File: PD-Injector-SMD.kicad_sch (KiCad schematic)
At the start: 10 parts

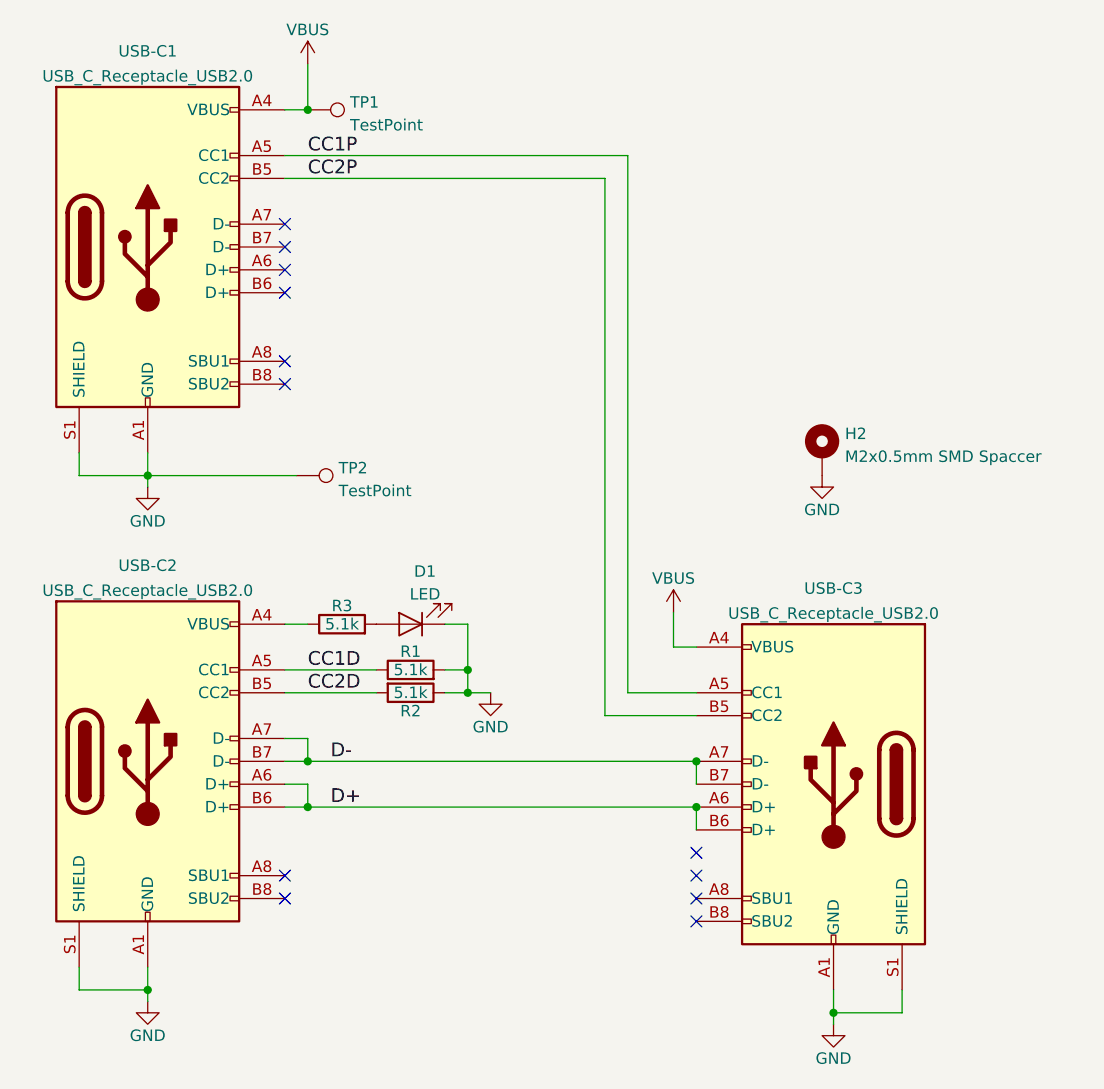
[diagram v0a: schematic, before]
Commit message: Update readme, minor mucking about
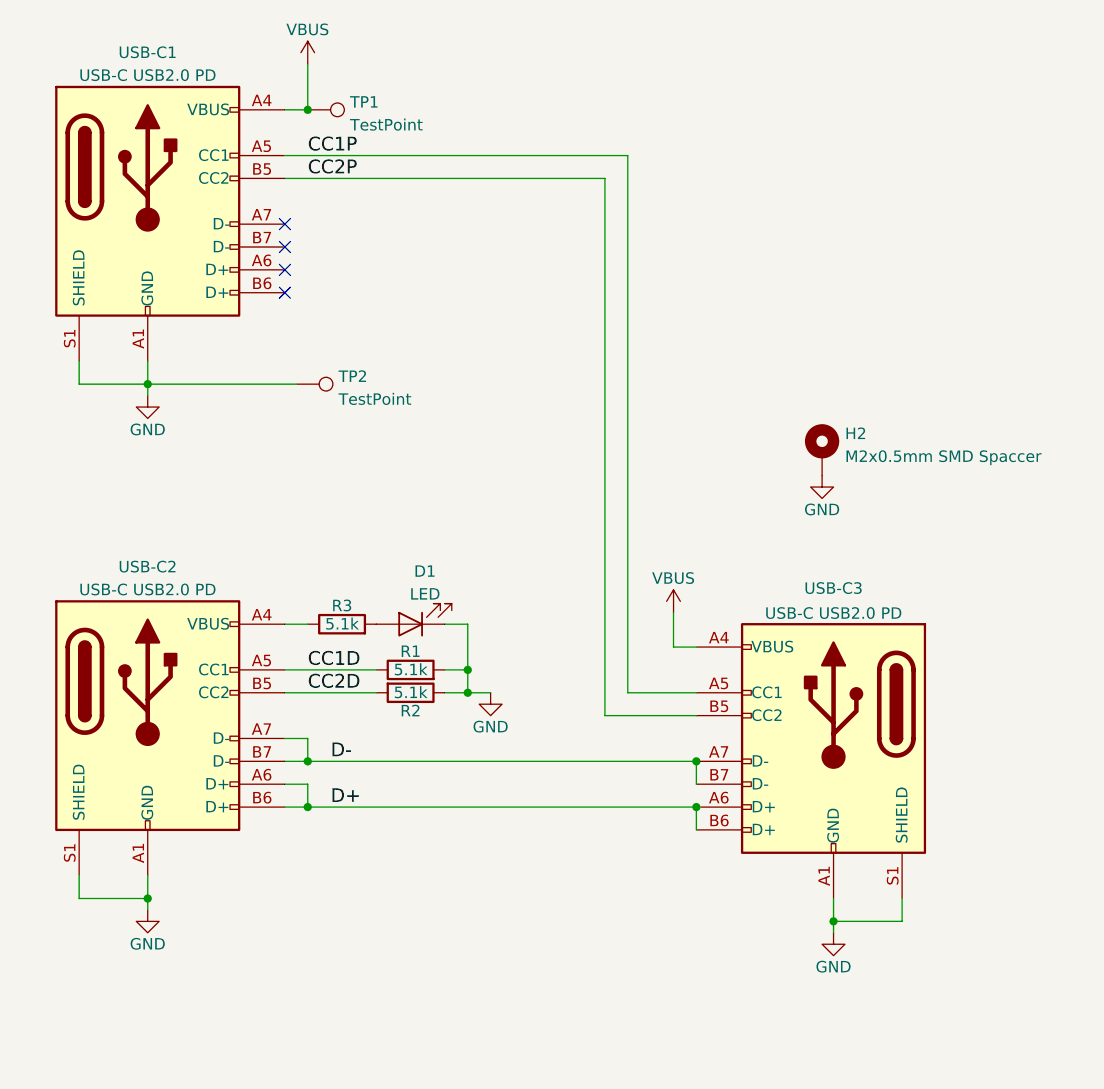
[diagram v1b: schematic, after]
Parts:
- USB-C1, USB-C2: value USB_C_Receptacle_USB2.0 -> USB-C USB2.0 PD; footprint Connector_USB_Extra:USB_C_Receptacle_GT-USB-7010 -> PD-Injector_SMD:USB_C_Receptacle_GT-USB-7010; symbol Connector:USB_C_Receptacle_USB2.0 -> PD-Injector-SMD:USB_C_Receptacle_USB2.0
- USB-C3: value USB_C_Receptacle_USB2.0 -> USB-C USB2.0 PD; symbol Connector:USB_C_Receptacle_USB2.0 -> PD-Injector-SMD:USB_C_Receptacle_USB2.0
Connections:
- net VBUS: now also USB-C3.A9 (VBUS), USB-C3.B4 (VBUS)
- net at R3.1, USB-C2.A4 (VBUS), USB-C2.B9 (VBUS): now also USB-C2.A9 (VBUS), USB-C2.B4 (VBUS)
- no-connect marks 12 -> 4
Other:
- moved on the sheet: TP2
